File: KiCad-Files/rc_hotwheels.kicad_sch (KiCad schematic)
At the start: 14 parts, among them IC1 BD6211F-E2, IC2 MIC5504-3.3YM5-TR, U1 STM32F070F6P6, U3 NRF24L01_Breakout

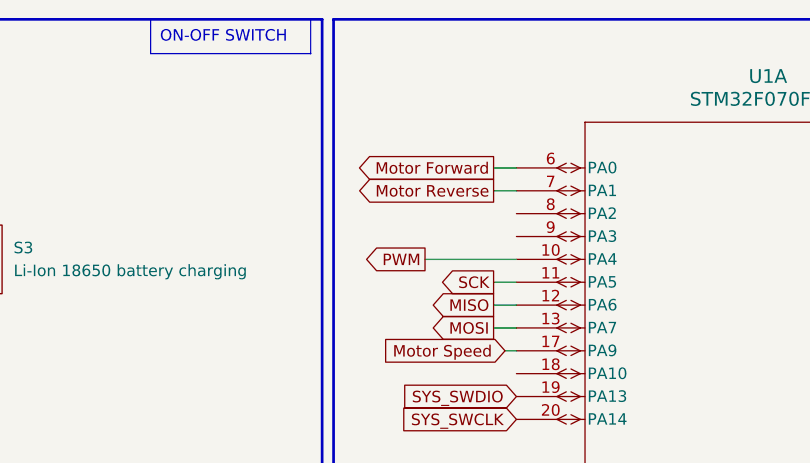
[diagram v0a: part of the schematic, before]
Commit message: PCB V2.0
Co-Authored-By: Yazid Almazroua <98489302+yazidta@users.noreply.github.com>
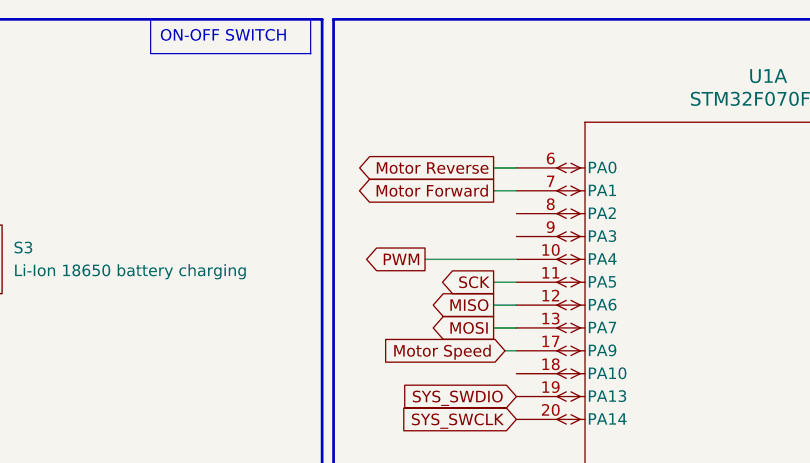
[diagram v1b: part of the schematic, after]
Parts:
- BT1: footprint (none) -> Library:Battery_Pads
- S3: footprint OS102011MA1QN1 -> Library:Battery_Pads
- SM1: footprint (none) -> Library:Servo_Motor
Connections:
- net Motor Forward: now also U1.7 (PA1); no longer U1.6 (PA0)
- net Motor Reverse: now also U1.6 (PA0); no longer U1.7 (PA1)
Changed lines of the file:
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@@
     )
   )
-  (global_label "Motor Reverse" (shape output) (at 208.28 33.02 180) (fields_autoplaced)
-    (effects (font (size 1.27 1.27)) (justify right))
-    (property "Intersheetrefs" "${INTERSHEET_REFS}" (at 191.7482 33.02 0)
-      (effects (font (size 1.27 1.27)) (justify right) hide)
-    )
-    (property "RIN" "" (at 208.28 35.2108 0)
+  (global_label "Motor Forward" (shape output) (at 208.28 33.02 180) (fields_autoplaced)
+    (effects (font (size 1.27 1.27)) (justify right))
+    (property "Intersheetrefs" "${INTERSHEET_REFS}" (at 191.6274 33.02 0)
+      (effects (font (size 1.27 1.27)) (justify right) hide)
+    )
+    (property "FIN" "" (at 208.28 35.2108 0)
       (effects (font (size 1.27 1.27)) (justify right) hide)
     )
@@
     )
   )
-  (global_label "Motor Forward" (shape output) (at 208.28 30.48 180) (fields_autoplaced)
-    (effects (font (size 1.27 1.27)) (justify right))
-    (property "Intersheetrefs" "${INTERSHEET_REFS}" (at 191.6274 30.48 0)
-      (effects (font (size 1.27 1.27)) (justify right) hide)
-    )
-    (property "FIN" "" (at 208.28 32.6708 0)
+  (global_label "Motor Reverse" (shape output) (at 208.28 30.48 180) (fields_autoplaced)
+    (effects (font (size 1.27 1.27)) (justify right))
+    (property "Intersheetrefs" "${INTERSHEET_REFS}" (at 191.7482 30.48 0)
+      (effects (font (size 1.27 1.27)) (justify right) hide)
+    )
+    (property "RIN" "" (at 208.28 32.6708 0)
       (effects (font (size 1.27 1.27)) (justify right) hide)
     )
@@
     (pin "1")
     (pin "2")
-    (pin "3")
     (pin "4")
     (pin "5")
+    (pin "3")
     (instances
       (project "rc_hotwheels"
@@
       (effects (font (size 1.27 1.27)) (justify left))
     )
-    (property "Footprint" "OS102011MA1QN1" (at 154.94 36.83 0)
+    (property "Footprint" "Library:Battery_Pads" (at 154.94 36.83 0)
       (effects (font (size 1.27 1.27)) (justify left) hide)
     )
@@
       (effects (font (size 1.27 1.27)) (justify left))
     )
-    (property "Footprint" "" (at 109.22 36.576 90)
+    (property "Footprint" "Library:Battery_Pads" (at 109.22 36.576 90)
       (effects (font (size 1.27 1.27)) hide)
     )
@@
       (effects (font (size 1.27 1.27)) (justify left))
     )
-    (property "Footprint" "" (at 62.23 128.016 0)
-      (effects (font (size 1.27 1.27)) hide)
-    )
+    (property "Footprint" "Library:Servo_Motor" (at 62.23 128.016 0)
+      (effects (font (size 1.27 1.27)) hide)
+    )
